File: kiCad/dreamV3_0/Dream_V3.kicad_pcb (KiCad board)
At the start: 2 copper layers, 80 x 80 mm, 44 parts, among them IC1 TGS2611-C00, J1 GPIO, J11 10132328-10011LF, J2 Qwiic_Vertical, J3 679305124022, J4 Qwiic_Vertical, J5 M20-7830542, J6 Qwiic_Vertical, J7 5013310607, J8 Qwiic_4pin_Vertical, J9 Qwiic_Vertical, Q1 BSS138, U1 AP2112K-3.3, U2 BME280, U3 INA219BxDCN, U5 BME280

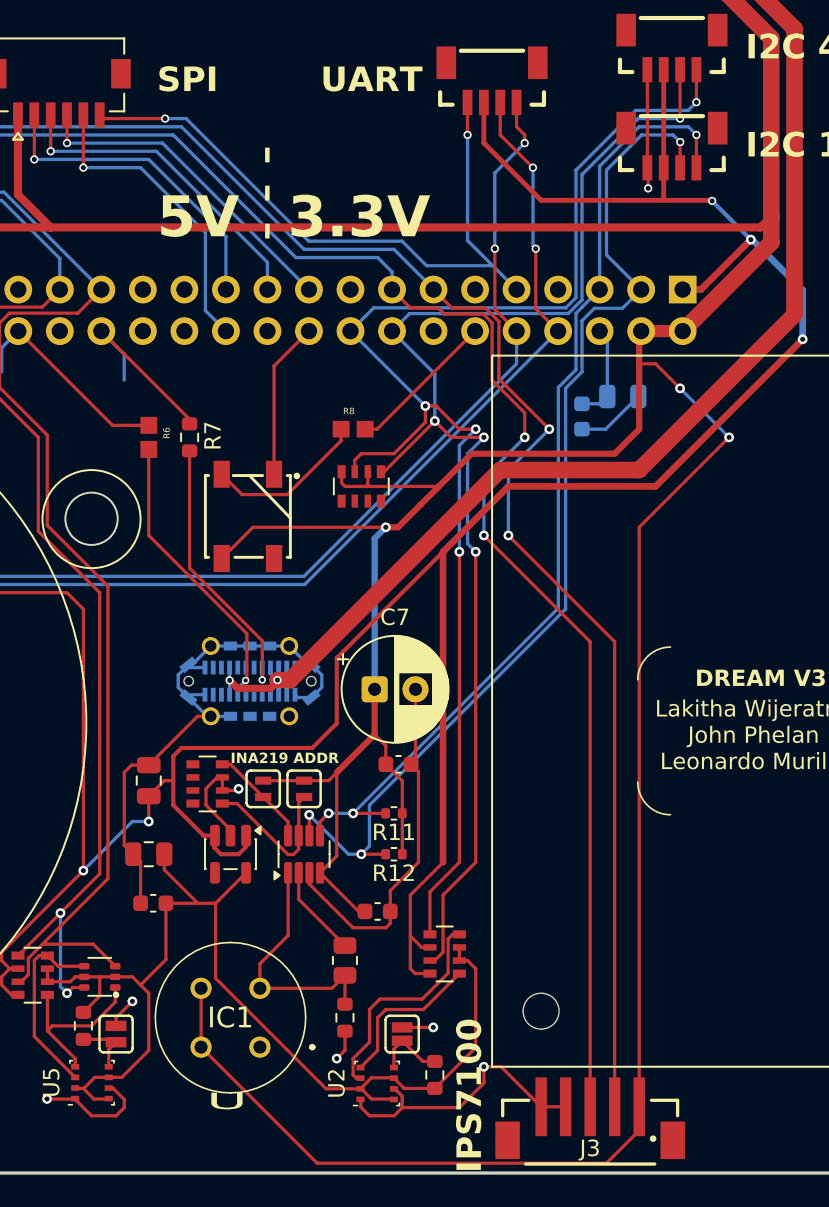
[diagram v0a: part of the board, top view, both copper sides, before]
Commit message: Final DreamV3
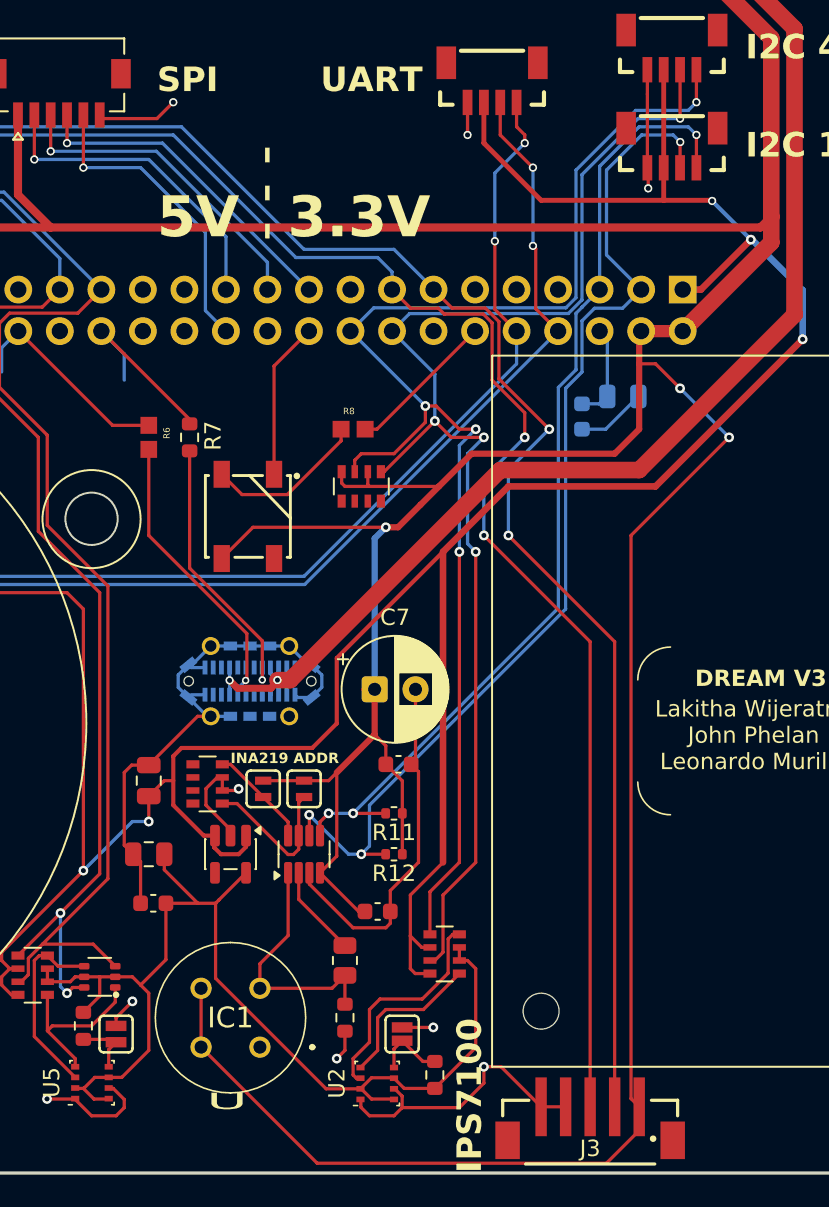
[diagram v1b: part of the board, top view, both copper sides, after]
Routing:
- net GND: track 207.3 -> 173.7 mm
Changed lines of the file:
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@@
 		(capping no)
 		(filling no)
+		(zone_defaults)
 		(pcbplotparams
 			(layerselection 0x00000000_00000000_55555555_5755f5ff)
@@
 		)
 	)
+	(dimension
+		(type orthogonal)
+		(layer "Dwgs.User")
+		(pts
+			(xy 55.5 96.5) (xy 129.5 96.5)
+		)
+		(height 8.5)
+		(orientation 0)
+		(format
+			(prefix "")
+			(suffix "")
+			(units 3)
+			(units_format 0)
+			(precision 4)
+			(suppress_zeroes yes)
+		)
+		(style
+			(thickness 0.1)
+			(arrow_length 1.27)
+			(text_position_mode 0)
+			(arrow_direction outward)
+			(extension_height 0.58642)
+			(extension_offset 0.5)
+			(keep_text_aligned yes)
+		)
+		(gr_text "74"
+			(at 92.5 103.85 0)
+			(layer "Dwgs.User")
+			(effects
+				(font
+					(size 1 1)
+					(thickness 0.15)
+				)
+			)
+		)
+	)
+	(dimension
+		(type orthogonal)
+		(layer "Dwgs.User")
+		(pts
+			(xy 55.5 22.5) (xy 55.5 96.5)
+		)
+		(height -9)
+		(orientation 1)
+		(format
+			(prefix "")
+			(suffix "")
+			(units 3)
+			(units_format 0)
+			(precision 4)
+			(suppress_zeroes yes)
+		)
+		(style
+			(thickness 0.1)
+			(arrow_length 1.27)
+			(text_position_mode 0)
+			(arrow_direction outward)
+			(extension_height 0.58642)
+			(extension_offset 0.5)
+			(keep_text_aligned yes)
+		)
+		(gr_text "74"
+			(at 45.35 59.5 90)
+			(layer "Dwgs.User")
+			(effects
+				(font
+					(size 1 1)
+					(thickness 0.15)
+				)
+			)
+		)
+	)
 	(segment
 		(start 114 98.4)
@@
 	)
 	(segment
-		(start 121.5 54)
-		(end 116 59.5)
-		(width 0.2)
-		(layer "F.Cu")
-		(net "+5V")
-	)
-	(segment
 		(start 80 41.16)
 		(end 69.66 41.16)
@@
 	)
 	(segment
+		(start 121.5 54)
+		(end 115.5 60)
+		(width 0.2)
+		(layer "F.Cu")
+		(net "+5V")
+	)
+	(segment
 		(start 98 57)
 		(end 97.8 56.8)
@@
 	)
 	(segment
+		(start 115.5 94.45)
+		(end 116 94.95)
+		(width 0.2)
+		(layer "F.Cu")
+		(net "+5V")
+	)
+	(segment
 		(start 116 94.95)
 		(end 116 96.4)
@@
 	)
 	(segment
+		(start 115.5 60)
+		(end 115.5 94.45)
+		(width 0.2)
+		(layer "F.Cu")
+		(net "+5V")
+	)
+	(segment
 		(start 93 75)
 		(end 95.5 75)
@@
 	)
 	(segment
-		(start 116 59.5)
-		(end 116 94.95)
-		(width 0.2)
-		(layer "F.Cu")
-		(net "+5V")
-	)
-	(segment
 		(start 117 22.5)
 		(end 124.08 29.58)
@@
 	)
 	(segment
+		(start 83.2175 34.5)
+		(end 83 34.2825)
+		(width 0.2)
+		(layer "F.Cu")
+		(net "GND")
+	)
+	(segment
 		(start 106.5 92.5)
 		(end 106.5 93.5)
@@
 	)
 	(segment
-		(start 83.2175 34.5)
-		(end 87 34.5)
-		(width 0.2)
-		(layer "F.Cu")
-		(net "GND")
-	)
-	(segment
 		(start 105.5 33.511)
 		(end 105.5 33.036)
@@
 	)
 	(segment
-		(start 83 34.2825)
-		(end 83.2175 34.5)
-		(width 0.2)
-		(layer "F.Cu")
-		(net "GND")
-	)
-	(segment
 		(start 84 95.5)
 		(end 84.5 95)
@@
 	)
 	(segment
+		(start 86.5 34.5)
+		(end 83.2175 34.5)
+		(width 0.2)
+		(layer "F.Cu")
+		(net "GND")
+	)
+	(segment
 		(start 66.5 31.511)
 		(end 66.5 37.511)
@@
 	)
 	(segment
+		(start 87.5 33.5)
+		(end 86.5 34.5)
+		(width 0.2)
+		(layer "F.Cu")
+		(net "GND")
+	)
+	(segment
 		(start 100.5 84)
 		(end 100.775 83.725)
@@
 	)
 	(via
-		(at 87 34.5)
+		(at 87.5 33.5)
 		(size 0.508)
 		(drill 0.3048)
@@
 	)
 	(segment
-		(start 88.284772 34.5)
-		(end 87 34.5)
-		(width 0.2)
-		(layer "B.Cu")
-		(net "GND")
-	)
-	(segment
-		(start 108.5 44.96)
-		(end 107.04 43.5)
-		(width 0.2)
-		(layer "B.Cu")
-		(net "GND")
-	)
-	(segment
 		(start 88.6435 67.9125)
 		(end 89.7935 66.7625)
@@
 	)
 	(segment
-		(start 107.04 43.5)
-		(end 103 43.5)
-		(width 0.2)
-		(layer "B.Cu")
-		(net "GND")
-	)
-	(segment
 		(start 92.1935 66.7625)
 		(end 90.9935 66.7625)
@@
 	)
 	(segment
-		(start 107.04 43.5)
-		(end 105.5 41.96)
-		(width 0.2)
-		(layer "B.Cu")
-		(net "GND")
-	)
-	(segment
 		(start 95.9635 67.9125)
 		(end 95.7435 67.9125)
@@
 	)
 	(segment
-		(start 103 43.5)
-		(end 101.5 42)
-		(width 0.2)
-		(layer "B.Cu")
-		(net "GND")
-	)
-	(segment
 		(start 114.05 51.5)
 		(end 114 51.5)
@@
 	)
 	(segment
-		(start 95.784772 42)
-		(end 88.284772 34.5)
-		(width 0.2)
-		(layer "B.Cu")
-		(net "GND")
-	)
-	(segment
 		(start 90.9935 71.0625)
 		(end 89.7935 71.0625)
@@
 	)
 	(segment
-		(start 101.5 42)
-		(end 95.784772 42)
-		(width 0.2)
-		(layer "B.Cu")
-		(net "GND")
-	)
-	(segment
-		(start 105.5 41.96)
-		(end 105.5 35.5)
-		(width 0.2)
-		(layer "B.Cu")
-		(net "GND")
-	)
-	(segment
 		(start 95.7935 68.0825)
 		(end 95.9635 67.9125)
@@
 	)
 	(segment
+		(start 109.672189 42.458642)
+		(end 109.672189 46.132189)
+		(width 0.2)
+		(layer "F.Cu")
+		(net "/GPIO14{slash}TXD0")
+	)
+	(segment
 		(start 60.5 61.5)
 		(end 60.58 61.42)
@@
 	)
 	(segment
-		(start 60.58 61.42)
-		(end 60.58 57)
+		(start 109.672189 46.132189)
+		(end 111.04 47.5)
 		(width 0.2)
 		(layer "F.Cu")
@@
 	)
 	(segment
-		(start 111.04 47.5)
-		(end 109.672189 46.132189)
+		(start 60.58 61.42)
+		(end 60.58 57)
 		(width 0.2)
 		(layer "F.Cu")
@@
 	)
 	(segment
-		(start 109.672189 46.132189)
+		(start 109.5 42.286453)
 		(end 109.672189 42.458642)
 		(width 0.2)
@@
 	)
 	(via
-		(at 109.672189 42.458642)
+		(at 109.5 42.286453)
 		(size 0.508)
 		(drill 0.3048)
@@
 	)
 	(segment
-		(start 109.672189 42.458642)
-		(end 109.5 42.286453)
-		(width 0.2)
-		(layer "B.Cu")
-		(net "/GPIO14{slash}TXD0")
-	)
-	(segment
 		(start 62 63)
 		(end 60.5 61.5)
@@
 	)
 	(segment
-		(start 109 35.5)
-		(end 108.5 35)
+		(start 107.171051 42)
+		(end 107.171051 46.171051)
 		(width 0.2)
 		(layer "F.Cu")
@@
 	)
 	(segment
-		(start 58.04 57)
-		(end 58.04 60.04)
+		(start 109 35.5)
+		(end 108.5 35)
 		(width 0.2)
 		(layer "F.Cu")
@@
 	)
 	(segment
-		(start 107.171051 46.171051)
-		(end 107.171051 42.458642)
+		(start 58.04 57)
+		(end 58.04 60.04)
 		(width 0.2)
 		(layer "F.Cu")
@@
 	)
 	(segment
-		(start 108.5 47.5)
-		(end 107.171051 46.171051)
+		(start 108.5 35)
+		(end 108.5 33.511)
 		(width 0.2)
 		(layer "F.Cu")
@@
 	)
 	(segment
-		(start 108.5 35)
-		(end 108.5 33.511)
+		(start 107.171051 46.171051)
+		(end 108.5 47.5)
 		(width 0.2)
 		(layer "F.Cu")
@@
 	)
 	(via
-		(at 107.171051 42.458642)
+		(at 107.171051 42)
 		(size 0.508)
 		(drill 0.3048)
@@
 	)
 	(segment
+		(start 107.171051 37.828949)
+		(end 109 36)
+		(width 0.2)
+		(layer "B.Cu")
+		(net "/GPIO15{slash}RXD0")
+	)
+	(segment
 		(start 95.5 62.5)
 		(end 108.5 49.5)
@@
 	)
 	(segment
-		(start 107.171051 37.828949)
-		(end 109 36)
+		(start 107.171051 42)
+		(end 107.171051 37.828949)
 		(width 0.2)
 		(layer "B.Cu")
@@
 		(width 0.2)
 		(layer "B.Cu")
-		(net "/GPIO15{slash}RXD0")
-	)
-	(segment
-		(start 107.171051 42.458642)
-		(end 107.171051 37.828949)
-		(width 0.2)
-		(layer "B.Cu")
